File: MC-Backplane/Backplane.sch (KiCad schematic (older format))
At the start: 6 parts

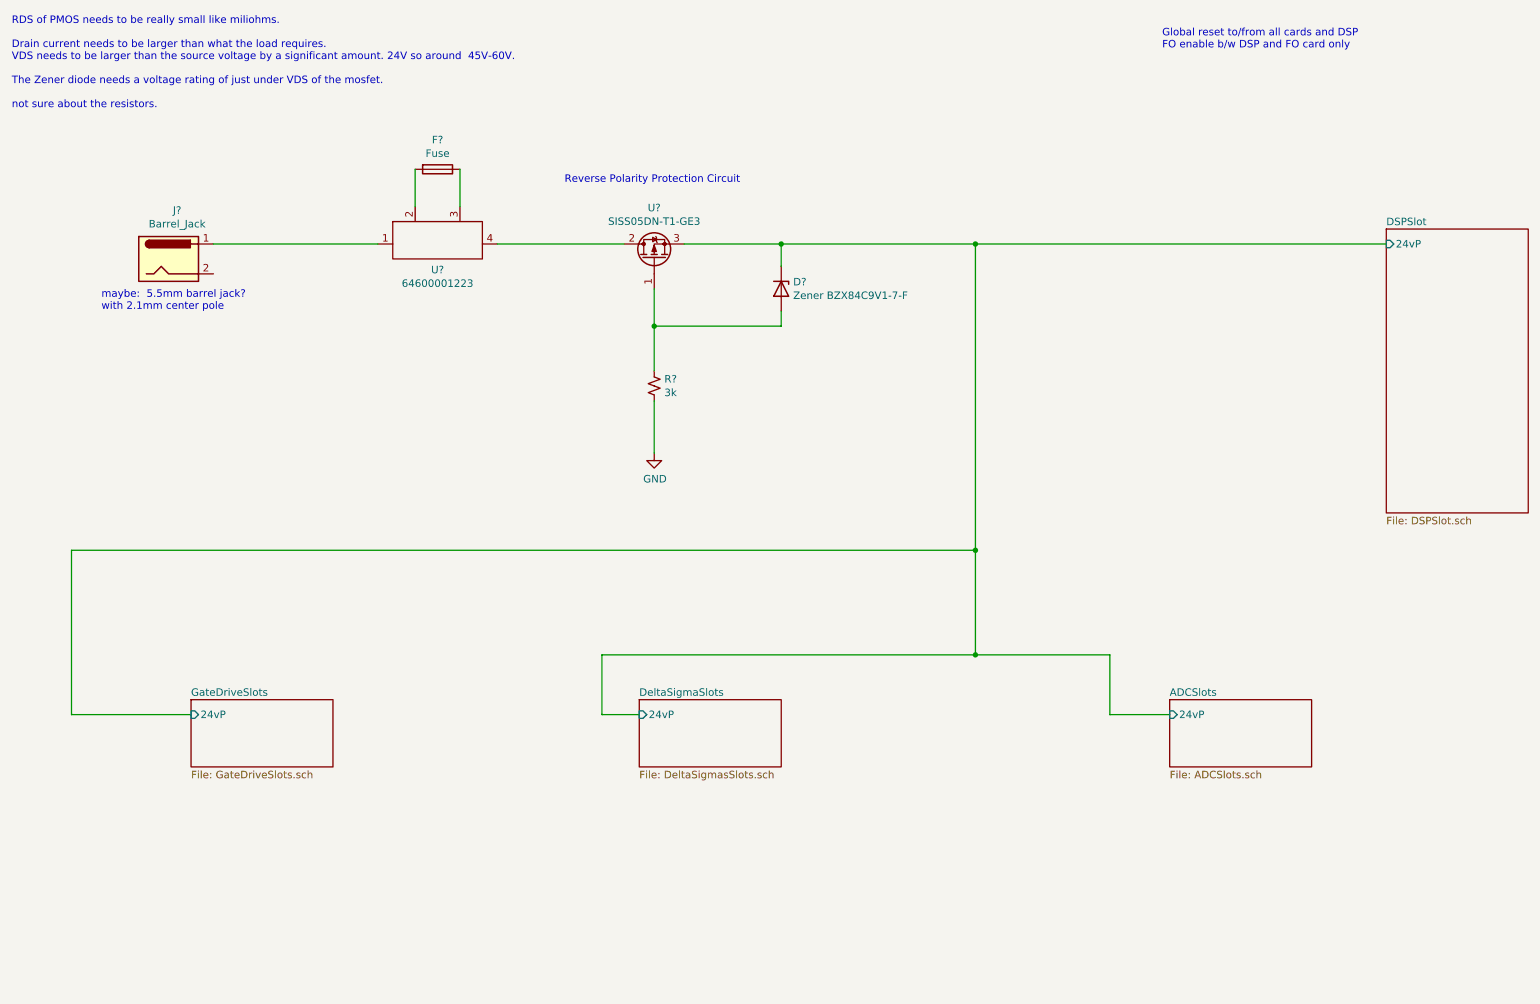
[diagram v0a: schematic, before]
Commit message: Add files via upload
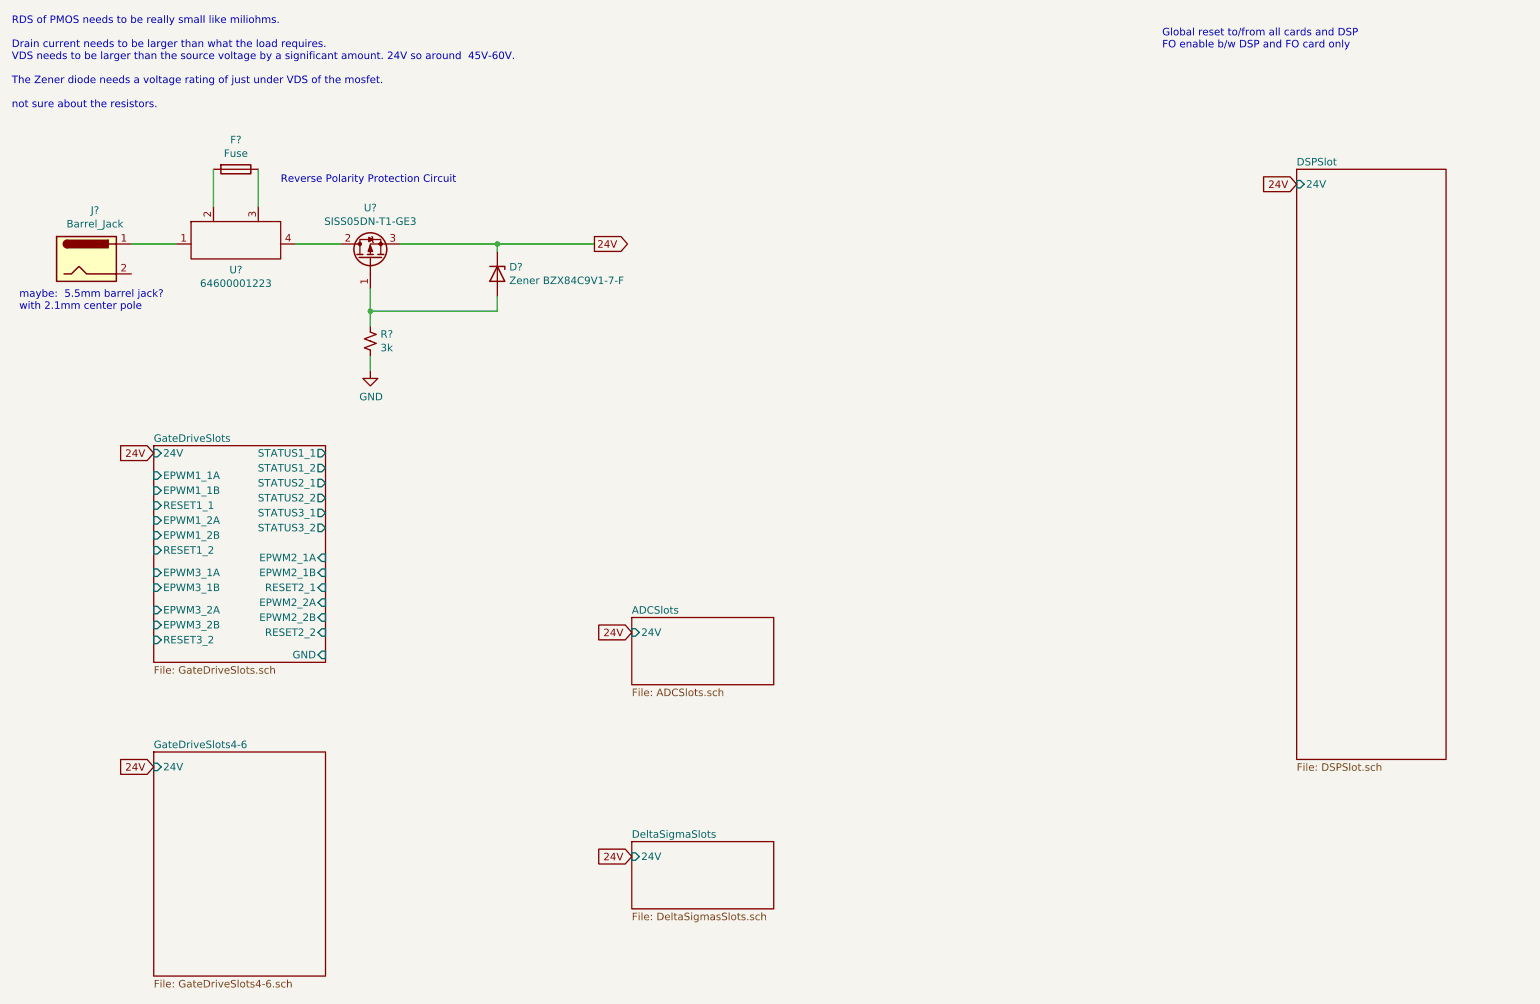
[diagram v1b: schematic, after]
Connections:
- net ADCSlots/24vP renamed 24V
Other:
- moved on the sheet: D?, F?, J?, R?, U?
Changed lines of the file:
@@
 $Descr A4 11693 8268
 encoding utf-8
-Sheet 1 5
+Sheet 1 6
 Title ""
 Date ""
@@
 $EndDescr
 $Sheet
-S 2000 5250 950  450
-U 61E8CAB3
-F0 "GateDriveSlots" 50
-F1 "GateDriveSlots.sch" 50
-F2 "24vP" I L 2000 5350 50
-$EndSheet
-$Sheet
-S 5000 5250 950  450
+S 4950 6200 950  450
 U 61E8CB73
 F0 "DeltaSigmaSlots" 50
 F1 "DeltaSigmasSlots.sch" 50
-F2 "24vP" I L 5000 5350 50
+F2 "24V" I L 4950 6300 50
 $EndSheet
 $Sheet
-S 8550 5250 950  450
+S 4950 4700 950  450
 U 61E8CB26
 F0 "ADCSlots" 50
 F1 "ADCSlots.sch" 50
-F2 "24vP" I L 8550 5350 50
+F2 "24V" I L 4950 4800 50
 $EndSheet
 $Comp
 L Device:D_Zener D?
 U 1 1 61EB8C1B
-P 5950 2500
-F 0 "D?" V 5904 2580 50  0000 L CNN
-F 1 "Zener BZX84C9V1-7-F" V 5995 2580 50  0000 L CNN
-F 2 "" H 5950 2500 50  0001 C CNN
-F 3 "https://www.digikey.com/en/products/detail/diodes-incorporated/BZX84C9V1-7-F/717755" H 5950 2500 50  0001 C CNN
-	1    5950 2500
+P 4050 2400
+F 0 "D?" V 4004 2480 50  0000 L CNN
+F 1 "Zener BZX84C9V1-7-F" V 4095 2480 50  0000 L CNN
+F 2 "" H 4050 2400 50  0001 C CNN
+F 3 "https://www.digikey.com/en/products/detail/diodes-incorporated/BZX84C9V1-7-F/717755" H 4050 2400 50  0001 C CNN
+	1    4050 2400
 	0    1    1    0
 $EndComp
@@
 L Device:R_Small_US R?
 U 1 1 61EBB5D2
-P 5100 3150
-F 0 "R?" H 5168 3196 50  0000 L CNN
-F 1 "3k" H 5168 3105 50  0000 L CNN
-F 2 "Resistor_SMD:R_1206_3216Metric" H 5100 3150 50  0001 C CNN
-F 3 "~" H 5100 3150 50  0001 C CNN
-	1    5100 3150
+P 3200 2850
+F 0 "R?" H 3268 2896 50  0000 L CNN
+F 1 "3k" H 3268 2805 50  0000 L CNN
+F 2 "Resistor_SMD:R_1206_3216Metric" H 3200 2850 50  0001 C CNN
+F 3 "~" H 3200 2850 50  0001 C CNN
+	1    3200 2850
 	1    0    0    -1
 $EndComp
 Wire Wire Line
-	5100 2500 5100 2750
+	3200 2500 3200 2650
 Wire Wire Line
-	5950 2650 5950 2750
+	4050 2550 4050 2650
 Wire Wire Line
-	5950 2750 5100 2750
-Connection ~ 5100 2750
+	4050 2650 3200 2650
+Connection ~ 3200 2650
 Wire Wire Line
-	5100 2750 5100 3050
+	3200 2650 3200 2750
 Wire Wire Line
-	5950 2350 5950 2200
+	4050 2250 4050 2200
 Wire Wire Line
-	5950 2200 5300 2200
-Connection ~ 5950 2200
+	4050 2200 3400 2200
 $Comp
 L power:GND #PWR0101
 U 1 1 61EBD36B
-P 5100 3600
-F 0 "#PWR0101" H 5100 3350 50  0001 C CNN
-F 1 "GND" H 5105 3427 50  0000 C CNN
-F 2 "" H 5100 3600 50  0001 C CNN
-F 3 "" H 5100 3600 50  0001 C CNN
-	1    5100 3600
+P 3200 3050
+F 0 "#PWR0101" H 3200 2800 50  0001 C CNN
+F 1 "GND" H 3205 2877 50  0000 C CNN
+F 2 "" H 3200 3050 50  0001 C CNN
+F 3 "" H 3200 3050 50  0001 C CNN
+	1    3200 3050
 	1    0    0    -1
 $EndComp
@@
 RDS of PMOS needs to be really small like miliohms.\n\nDrain current needs to be larger than what the load requires.\nVDS needs to be larger than the source voltage by a significant amount. 24V so around  45V-60V.\n\nThe Zener diode needs a voltage rating of just under VDS of the mosfet. \n\nnot sure about the resistors.
 Wire Wire Line
-	5100 3250 5100 3600
-Text Notes 4500 1800 0    50   ~ 0
+	3200 2950 3200 3050
+Text Notes 2600 1800 0    50   ~ 0
 Reverse Polarity Protection Circuit
 Text Notes 8500 900  0    50   ~ 0
 Global reset to/from all cards and DSP\nFO enable b/w DSP and FO card only
-Wire Wire Line
-	1200 4250 1200 5350
-Wire Wire Line
-	1200 5350 2000 5350
-Wire Wire Line
-	4750 5350 5000 5350
-Wire Wire Line
-	4750 4950 7250 4950
-Wire Wire Line
-	8150 4950 8150 5350
-Wire Wire Line
-	8150 5350 8550 5350
-Wire Wire Line
-	4750 4950 4750 5350
 $Comp
 L MC-Backplane:64600001223 U?
 U 1 1 61F13696
-P 3650 2400
-F 0 "U?" H 3650 2427 50  0000 C CNN
-F 1 "64600001223" H 3650 2336 50  0000 C CNN
-F 2 "" H 3650 2400 50  0001 C CNN
-F 3 "https://www.littelfuse.com/~/media/electronics/datasheets/fuse_blocks/littelfuse_fuse_block_646_datasheet.pdf.pdf" H 3650 2400 50  0001 C CNN
-	1    3650 2400
+P 2300 2400
+F 0 "U?" H 2300 2427 50  0000 C CNN
+F 1 "64600001223" H 2300 2336 50  0000 C CNN
+F 2 "" H 2300 2400 50  0001 C CNN
+F 3 "https://www.littelfuse.com/~/media/electronics/datasheets/fuse_blocks/littelfuse_fuse_block_646_datasheet.pdf.pdf" H 2300 2400 50  0001 C CNN
+	1    2300 2400
 	1    0    0    -1
 $EndComp
 Wire Wire Line
-	4050 2200 4900 2200
-Wire Wire Line
-	5950 2200 7250 2200
-Wire Wire Line
-	1200 4250 7250 4250
-Wire Wire Line
-	7250 4250 7250 2200
-Connection ~ 7250 2200
-Wire Wire Line
-	7250 2200 10000 2200
-Wire Wire Line
-	7250 4250 7250 4950
-Connection ~ 7250 4250
-Connection ~ 7250 4950
-Wire Wire Line
-	7250 4950 8150 4950
+	2700 2200 3000 2200
 $Comp
 L Connector:Barrel_Jack J?
 U 1 1 61F21CB0
-P 1850 2300
-F 0 "J?" H 1907 2625 50  0000 C CNN
-F 1 "Barrel_Jack" H 1907 2534 50  0000 C CNN
-F 2 "" H 1900 2260 50  0001 C CNN
-F 3 "~" H 1900 2260 50  0001 C CNN
-	1    1850 2300
+P 1300 2300
+F 0 "J?" H 1357 2625 50  0000 C CNN
+F 1 "Barrel_Jack" H 1357 2534 50  0000 C CNN
+F 2 "" H 1350 2260 50  0001 C CNN
+F 3 "~" H 1350 2260 50  0001 C CNN
+	1    1300 2300
 	1    0    0    -1
 $EndComp
 Wire Wire Line
-	2150 2200 3250 2200
+	1600 2200 1900 2200
 $Comp
 L Device:Fuse F?
 U 1 1 61F2B17A
-P 3650 1700
-F 0 "F?" V 3453 1700 50  0000 C CNN
-F 1 "Fuse" V 3544 1700 50  0000 C CNN
-F 2 "" V 3580 1700 50  0001 C CNN
-F 3 "~" H 3650 1700 50  0001 C CNN
-	1    3650 1700
+P 2300 1700
+F 0 "F?" V 2103 1700 50  0000 C CNN
+F 1 "Fuse" V 2194 1700 50  0000 C CNN
+F 2 "" V 2230 1700 50  0001 C CNN
+F 3 "~" H 2300 1700 50  0001 C CNN
+	1    2300 1700
 	0    1    1    0
 $EndComp
 Wire Wire Line
-	3500 1700 3500 1950
+	2150 1700 2150 1950
 Wire Wire Line
-	3800 1950 3800 1700
-Text Notes 1400 2650 0    50   ~ 0
+	2450 1950 2450 1700
+Text Notes 850  2650 0    50   ~ 0
 maybe:  5.5mm barrel jack? \nwith 2.1mm center pole
 $Comp
 L MC-Backplane:SISS05DN-T1-GE3 U?
 U 1 1 61F2E911
-P 5600 2200
-F 0 "U?" V 5842 2700 50  0000 C CNN
-F 1 "SISS05DN-T1-GE3" V 5751 2700 50  0000 C CNN
-F 2 "" H 5600 2200 50  0001 C CNN
-F 3 "" H 5600 2200 50  0001 C CNN
-	1    5600 2200
+P 3700 2200
+F 0 "U?" V 3942 2700 50  0000 C CNN
+F 1 "SISS05DN-T1-GE3" V 3851 2700 50  0000 C CNN
+F 2 "" H 3700 2200 50  0001 C CNN
+F 3 "" H 3700 2200 50  0001 C CNN
+	1    3700 2200
 	0    -1   -1   0
 $EndComp
 $Sheet
-S 10000 2100 950  1900
+S 9400 1700 1000 3950
 U 61E8CBE3
 F0 "DSPSlot" 50
 F1 "DSPSlot.sch" 50
-F2 "24vP" I L 10000 2200 50
+F2 "24V" I L 9400 1800 50
 $EndSheet
+$Sheet
+S 1750 3550 1150 1450
+U 61E8CAB3
+F0 "GateDriveSlots" 50
+F1 "GateDriveSlots.sch" 50
+F2 "24V" I L 1750 3600 50
+F3 "GND" I R 2900 4950 50
+F4 "EPWM1_1A" I L 1750 3750 50
+F5 "EPWM1_1B" I L 1750 3850 50
+F6 "RESET1_1" I L 1750 3950 50
+F7 "STATUS1_1" O R 2900 3600 50
+F8 "EPWM1_2A" I L 1750 4050 50
+F9 "EPWM1_2B" I L 1750 4150 50
+F10 "RESET1_2" I L 1750 4250 50
+F11 "STATUS1_2" O R 2900 3700 50
+F12 "EPWM3_1A" I L 1750 4400 50
+F13 "EPWM3_1B" I L 1750 4500 50
+F14 "STATUS3_1" O R 2900 4000 50
+F15 "EPWM3_2A" I L 1750 4650 50
+F16 "EPWM3_2B" I L 1750 4750 50
+F17 "RESET3_2" I L 1750 4850 50
+F18 "EPWM2_1A" I R 2900 4300 50
+F19 "EPWM2_1B" I R 2900 4400 50
+F20 "RESET2_1" I R 2900 4500 50
+F21 "STATUS2_1" O R 2900 3800 50
+F22 "EPWM2_2A" I R 2900 4600 50
+F23 "EPWM2_2B" I R 2900 4700 50
+F24 "RESET2_2" I R 2900 4800 50
+F25 "STATUS2_2" O R 2900 3900 50
+F26 "STATUS3_2" O R 2900 4100 50
+$EndSheet
+$Sheet
+S 1750 5600 1150 1500
+U 61F59C33
+F0 "GateDriveSlots4-6" 50
+F1 "GateDriveSlots4-6.sch" 50
+F2 "24V" I L 1750 5700 50
+$EndSheet
+Wire Wire Line
+	4050 2200 4700 2200
+Connection ~ 4050 2200
+Text GLabel 4700 2200 2    50   Output ~ 0
+24V
+Text GLabel 1750 3600 0    50   Input ~ 0
+24V
+Text GLabel 1750 5700 0    50   Input ~ 0
+24V
+Text GLabel 4950 6300 0    50   Input ~ 0
+24V
+Text GLabel 4950 4800 0    50   Input ~ 0
+24V
+Text GLabel 9400 1800 0    50   Input ~ 0
+24V
 $EndSCHEMATC
